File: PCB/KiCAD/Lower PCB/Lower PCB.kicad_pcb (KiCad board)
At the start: 2 copper layers, 188.6 x 165.4 mm, 106 parts, among them IC1 ADG608BRZ, IC2 ADG608BRZ, IC3 ADG608BRZ, J1 Conn_01x02_MountingPin, J2 Conn_01x04_MountingPin, J3 Conn_01x04_MountingPin, J4 Conn_01x04_MountingPin, Q1 SFH320, Q10 SFH320, Q11 SFH320, Q12 SFH320, Q13 SFH320, Q14 SFH320, Q15 SFH320, Q16 SFH320, Q17 SFH320, Q18 SFH320, Q19 SFH320, Q2 SFH320, Q20 SFH320, Q21 SFH320, Q22 SFH320, Q23 SFH320, Q24 SFH320, Q3 SFH320, Q4 SFH320, Q5 SFH320, Q6 SFH320, Q7 SFH320, Q8 SFH320, Q9 SFH320

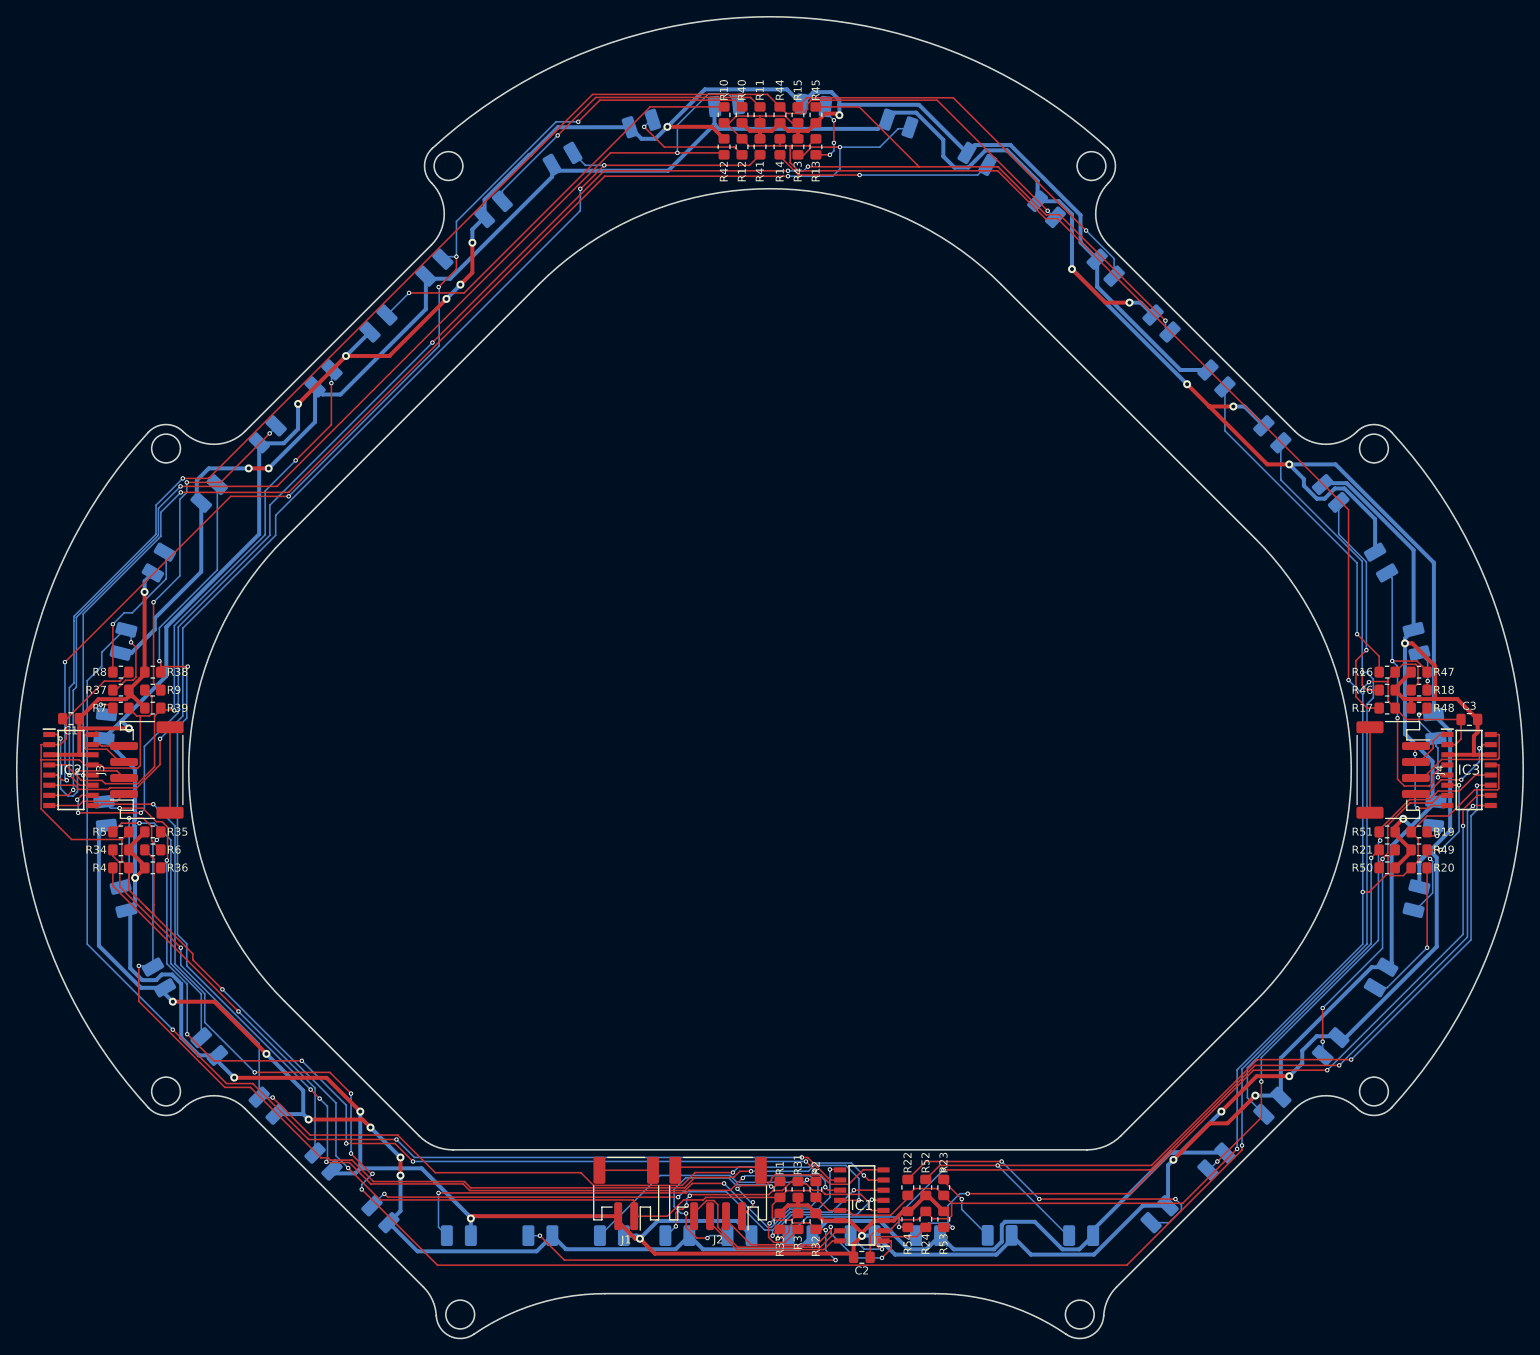
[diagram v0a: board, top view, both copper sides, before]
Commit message: Uh oh there was a +5V rail
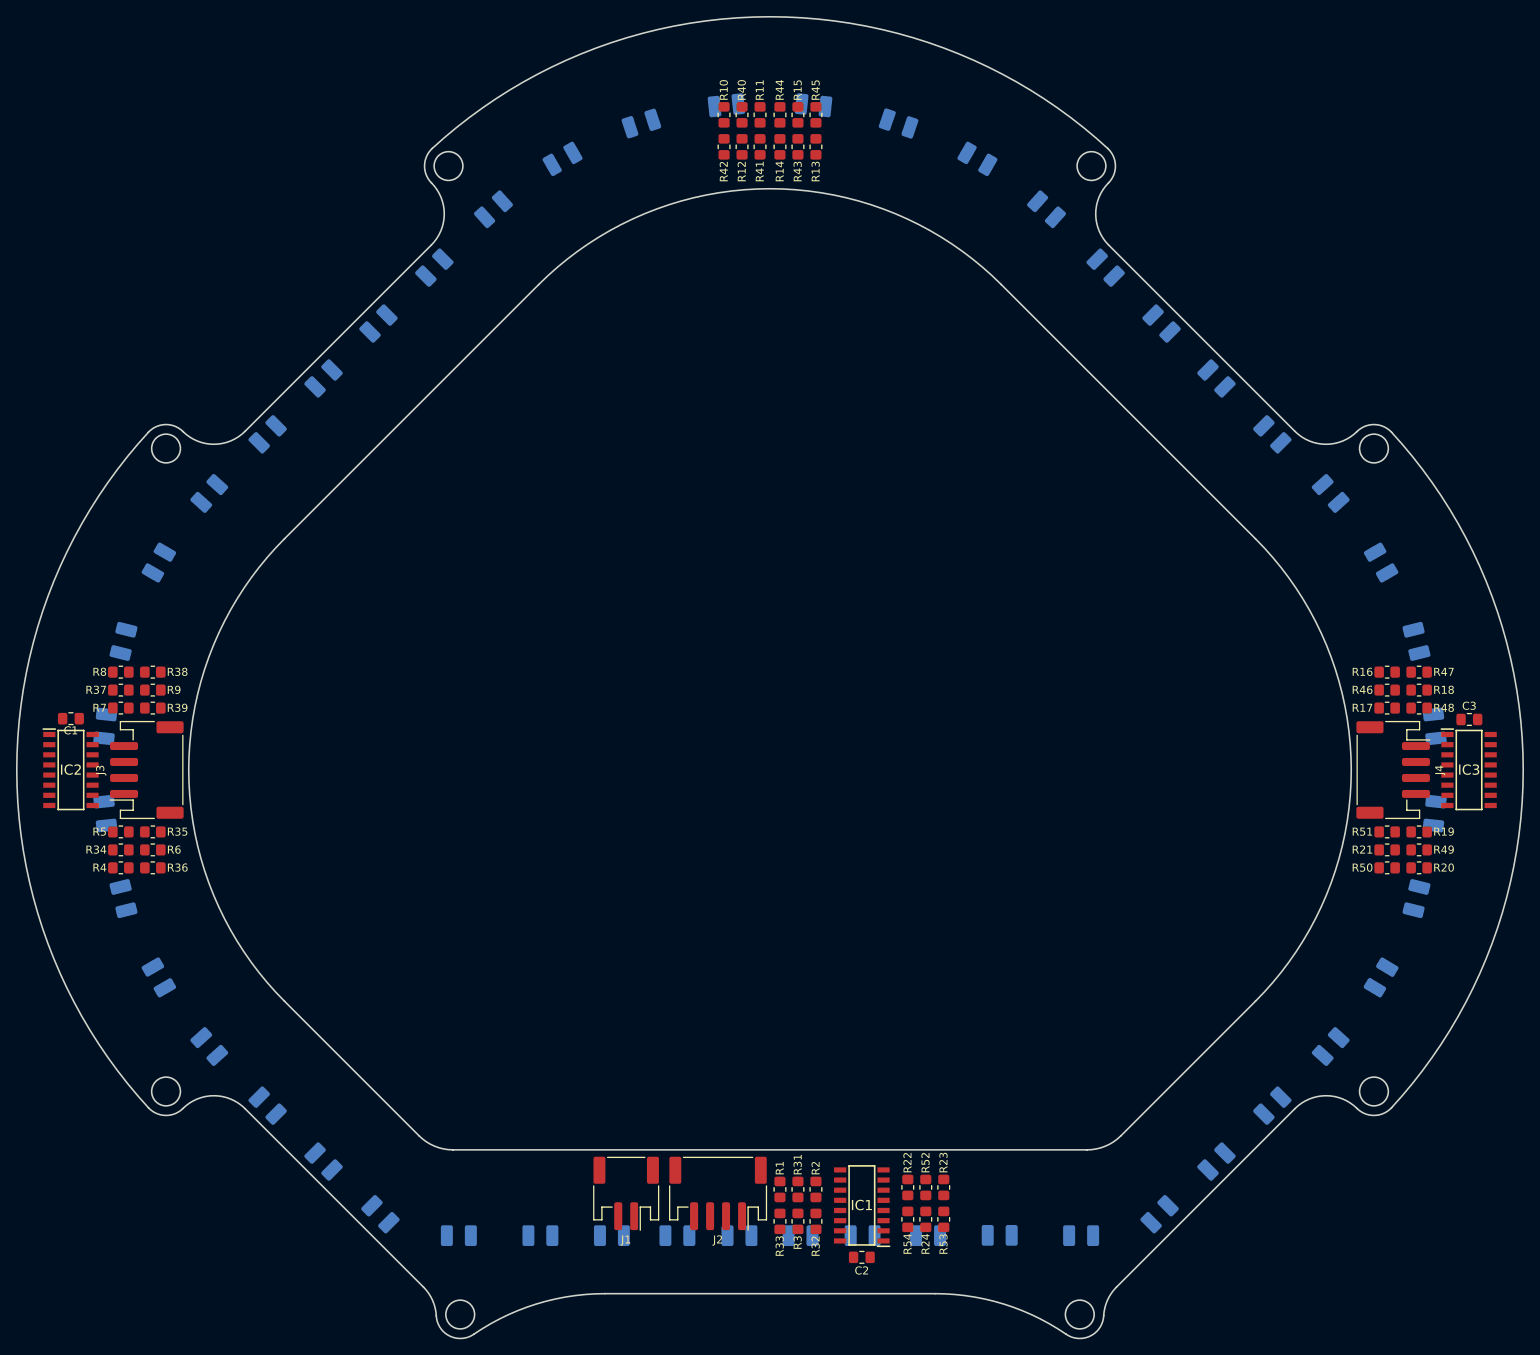
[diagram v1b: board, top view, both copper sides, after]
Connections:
- Q1 pad 1: +5V -> +3V3
- Q10 pad 1: +5V -> +3V3
- Q11 pad 1: +5V -> +3V3
- Q12 pad 1: +5V -> +3V3
- Q13 pad 1: +5V -> +3V3
- Q14 pad 1: +5V -> +3V3
- Q15 pad 1: +5V -> +3V3
- Q16 pad 1: +5V -> +3V3
- Q17 pad 1: +5V -> +3V3
- Q18 pad 1: +5V -> +3V3
- Q19 pad 1: +5V -> +3V3
- Q2 pad 1: +5V -> +3V3
- Q20 pad 1: +5V -> +3V3
- Q21 pad 1: +5V -> +3V3
- Q22 pad 1: +5V -> +3V3
- Q23 pad 1: +5V -> +3V3
- Q24 pad 1: +5V -> +3V3
- Q3 pad 1: +5V -> +3V3
- Q4 pad 1: +5V -> +3V3
- Q5 pad 1: +5V -> +3V3
- Q6 pad 1: +5V -> +3V3
- Q7 pad 1: +5V -> +3V3
- Q8 pad 1: +5V -> +3V3
- Q9 pad 1: +5V -> +3V3
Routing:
- net GND: track 702.4 -> 0.00 mm, vias 19 -> 0
- net +5V: track 587.0 -> 0.00 mm, vias 15 -> 0
- net +3V3: track 535.4 -> 0.00 mm, vias 6 -> 0
- net Net-(IC2-S8): track 297.9 -> 0.00 mm, vias 8 -> 0
- net Net-(IC2-S7): track 212.2 -> 0.00 mm, vias 7 -> 0
- net Net-(IC2-S6): track 183.7 -> 0.00 mm, vias 3 -> 0
- net Net-(IC1-S8): track 174.9 -> 0.00 mm, vias 7 -> 0
- net Net-(IC2-S5): track 159.1 -> 0.00 mm, vias 4 -> 0
- net Net-(IC1-S7): track 158.0 -> 0.00 mm, vias 4 -> 0
- net Net-(IC2-S4): track 145.6 -> 0.00 mm, vias 3 -> 0
- net Net-(IC2-S2): track 141.3 -> 0.00 mm, vias 6 -> 0
- net Net-(IC2-S3): track 138.1 -> 0.00 mm, vias 3 -> 0
- net Net-(IC1-S6): track 130.6 -> 0.00 mm, vias 9 -> 0
- net Net-(IC1-S5): track 130.3 -> 0.00 mm, vias 4 -> 0
- net Net-(IC1-S4): track 123.3 -> 0.00 mm, vias 4 -> 0
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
